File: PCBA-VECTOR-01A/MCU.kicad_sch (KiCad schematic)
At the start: 24 parts, among them J12 Conn_02x03_Odd_Even, U11 STM32G473RCTx, Y1 25MHz, Y2 32.768kHz

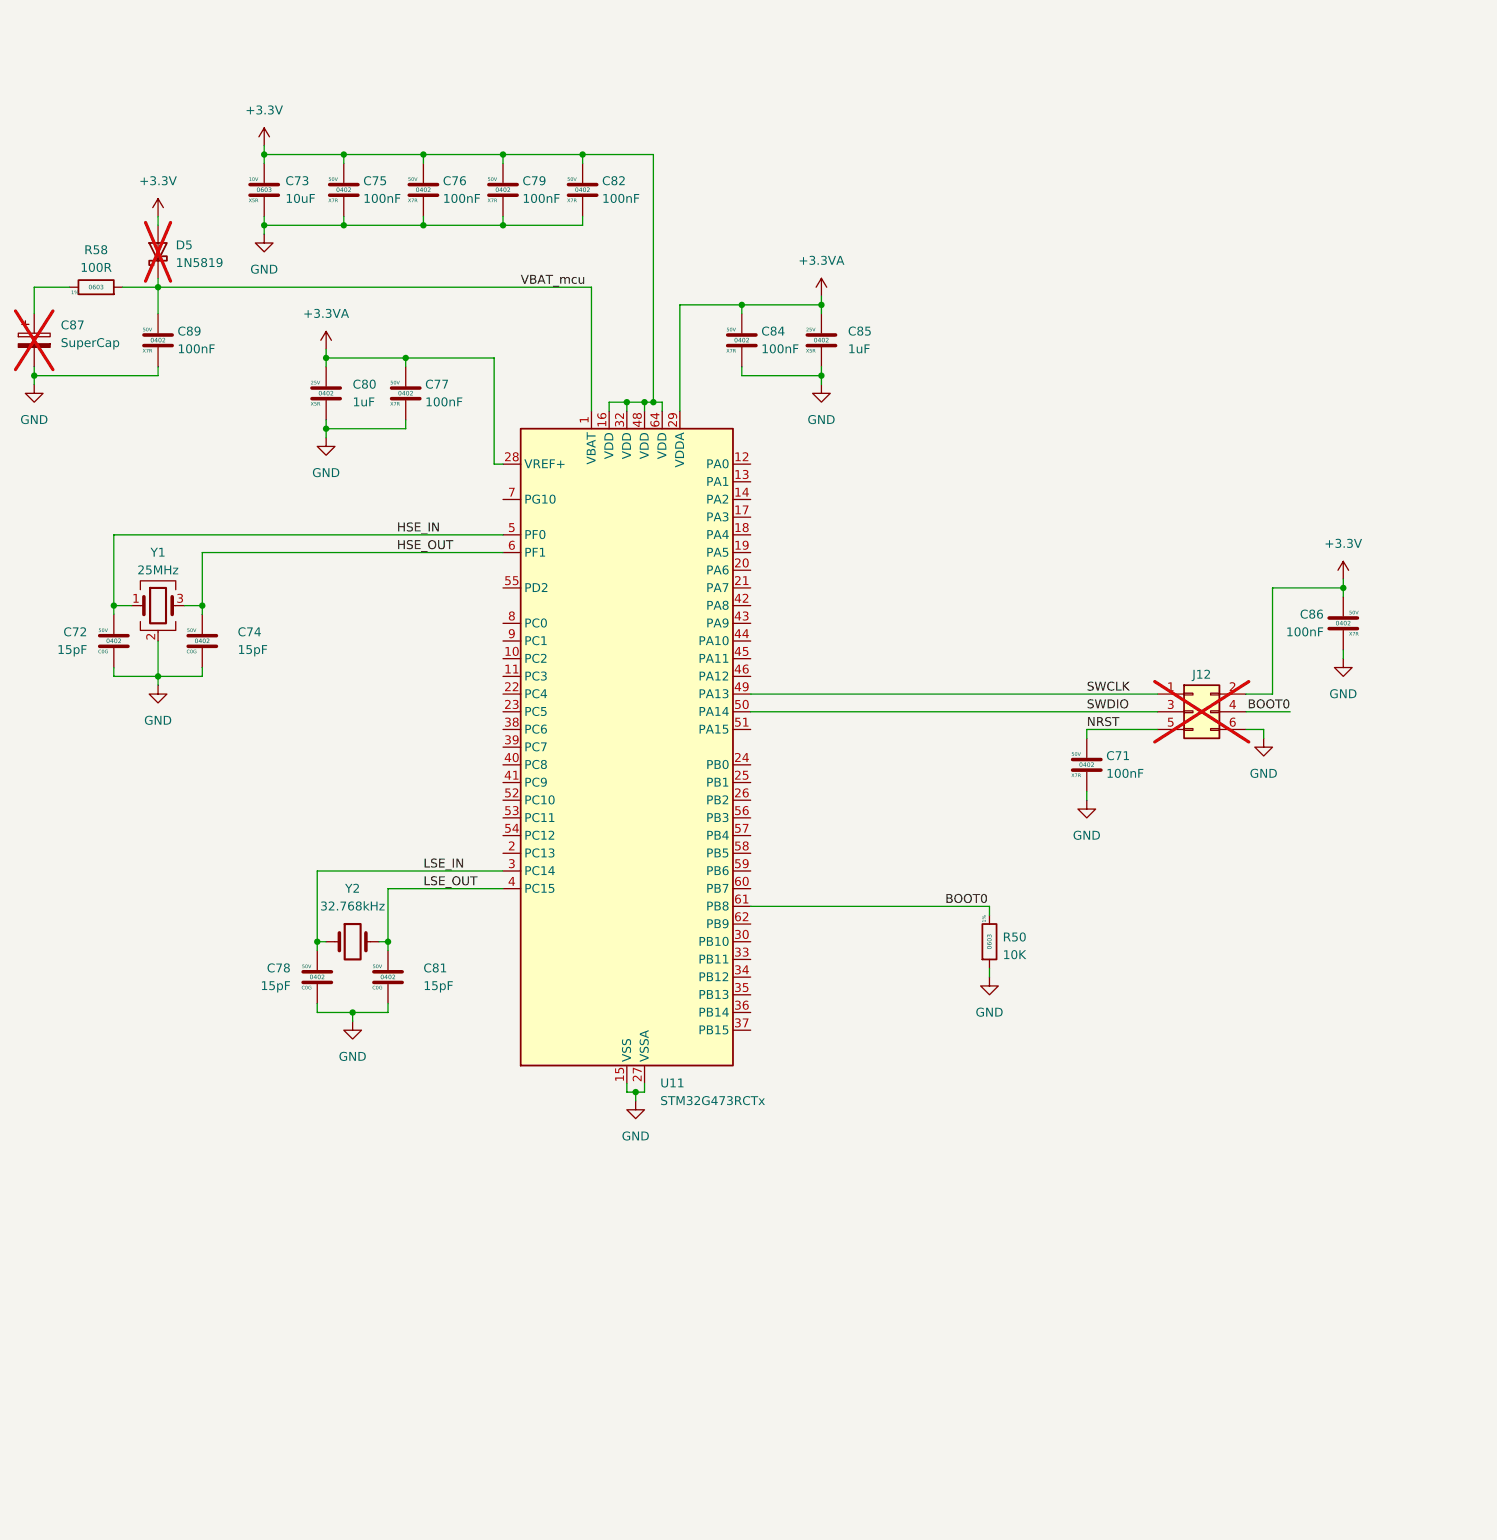
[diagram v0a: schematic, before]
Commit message: Changes were made
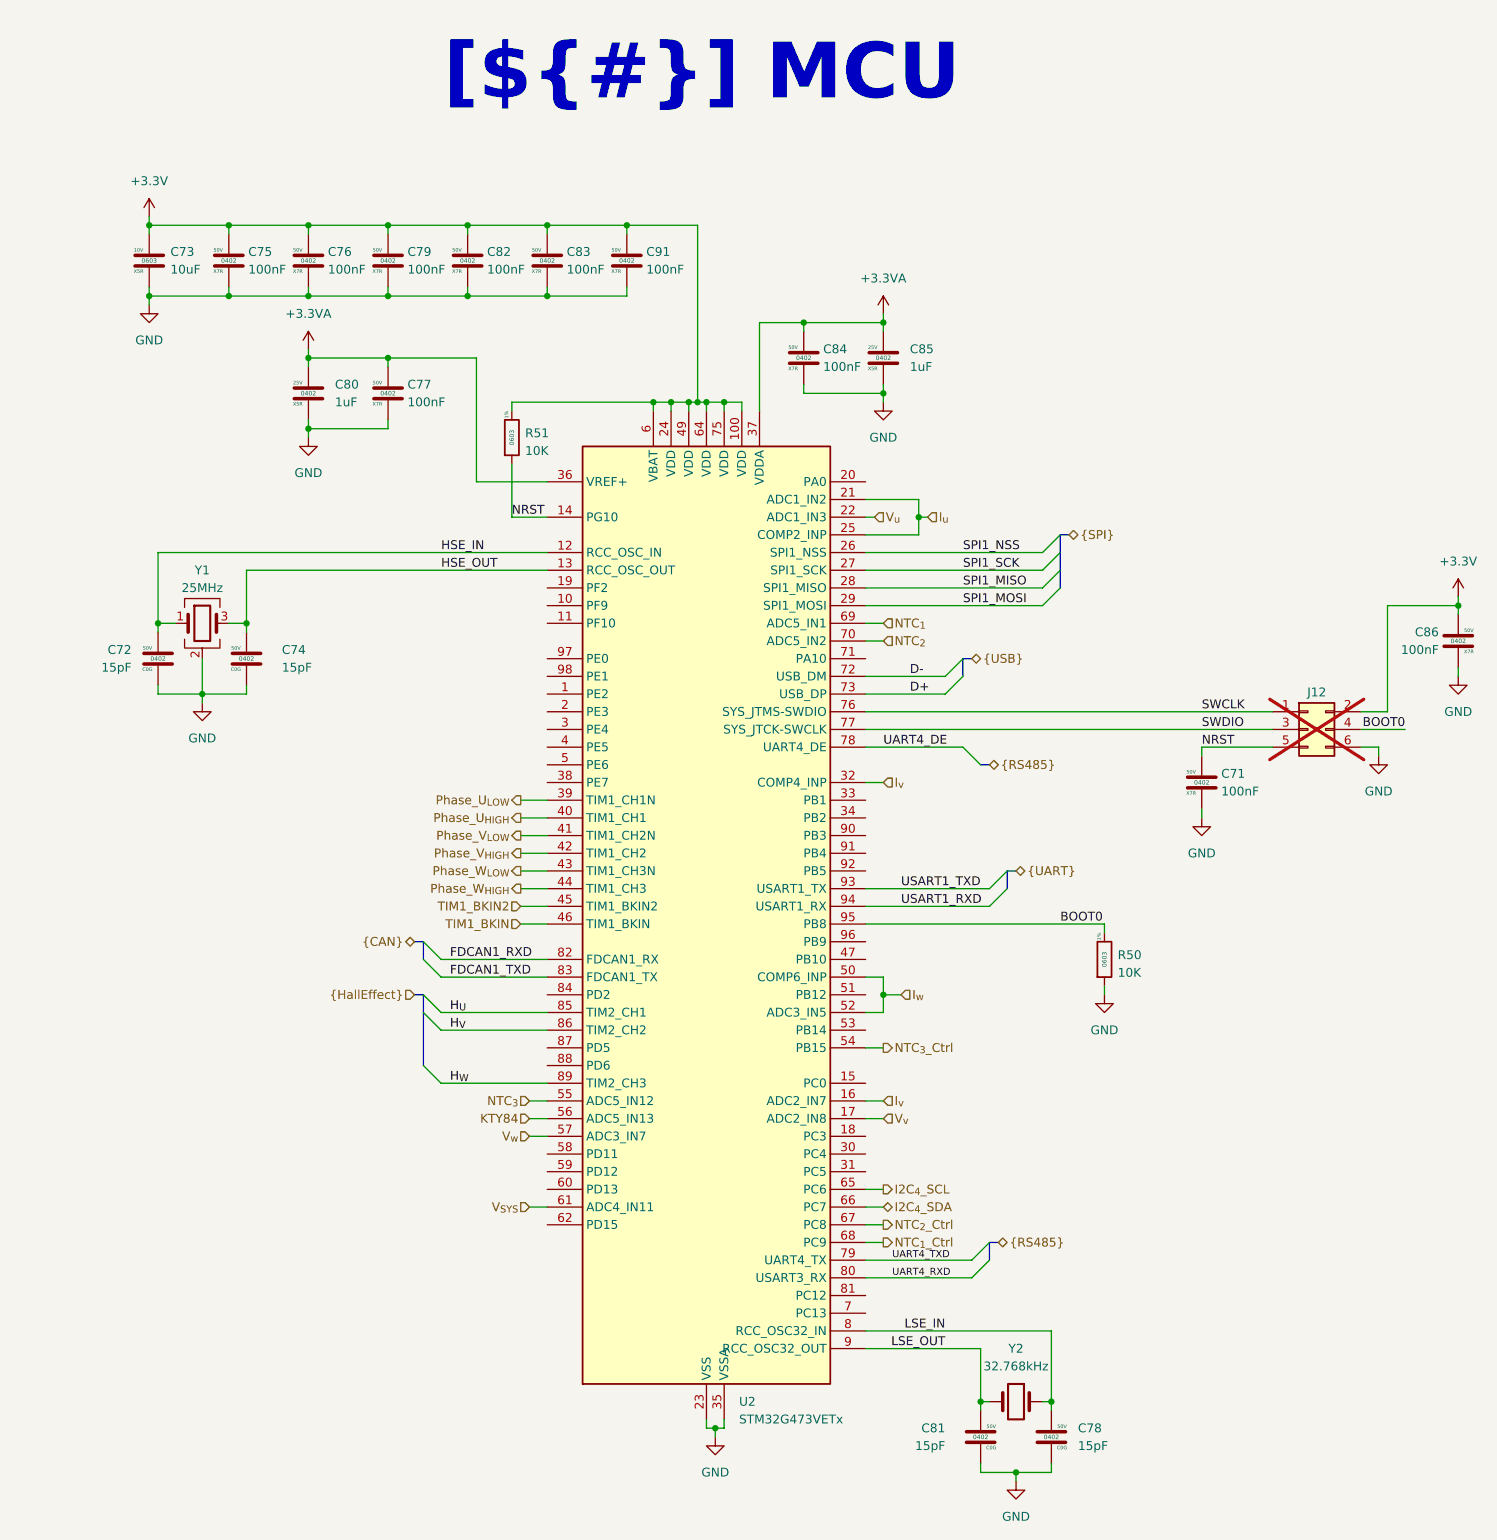
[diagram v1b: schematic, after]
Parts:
- removed C87: SuperCap, Capacitor_THT:C_Rect_L7.2mm_W11.0mm_P5.00mm_FKS2_FKP2_MKS2_MKP2, symbol Device:C_Polarized
- removed C89: 100nF, Capacitor_SMD:C_0402_1005Metric, symbol Device:C
- removed D5: 1N5819, Diode_THT:D_DO-41_SOD81_P10.16mm_Horizontal, symbol Diode:1N5819
- removed R58: 100R, Resistor_SMD:R_0603_1608Metric, symbol Device:R
- removed U11: STM32G473RCTx, Package_QFP:LQFP-64_10x10mm_P0.5mm, symbol MCU_ST_STM32G4:STM32G473RCTx
- added C83, C91: 100nF, Capacitor_SMD:C_0402_1005Metric, symbol Device:C
- added R51: 10K, Resistor_SMD:R_0603_1608Metric, symbol Device:R
- added U2: STM32G473VETx, Package_QFP:LQFP-100_14x14mm_P0.5mm, symbol MCU_ST_STM32G4:STM32G473VETx
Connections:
- net +3.3V: now also C83.1, C91.1, R51.1, U2.100 (VDD), U2.24 (VDD), U2.49 (VDD), U2.6 (VBAT), U2.64 (VDD), U2.75 (VDD)
- net +3.3VA: now also U2.36 (VREF+), U2.37 (VDDA)
- net BOOT0: now also U2.95 (PB8)
- net GND: now also C83.2, C91.2, U2.23 (VSS), U2.35 (VSSA), U2.48 (VSS), U2.63 (VSS), U2.74 (VSS), U2.99 (VSS)
- net HSE_IN: now also U2.12 (PF0)
- net HSE_OUT: now also U2.13 (PF1)
- net LSE_IN: now also U2.8 (PC14)
- net LSE_OUT: now also U2.9 (PC15)
- net NRST: now also R51.2, U2.14 (PG10)
- net SWCLK: now also U2.76 (PA13)
- net SWDIO: now also U2.77 (PA14)
- new net D+: U2.73 (PA12)
- new net D-: U2.72 (PA11)
- new net FDCAN1_RXD: U2.82 (PD0)
- new net FDCAN1_TXD: U2.83 (PD1)
- new net H_{U}: U2.85 (PD3)
- new net H_{V}: U2.86 (PD4)
- new net H_{W}: U2.89 (PD7)
- new net I2C_{4}_SCL: U2.65 (PC6)
- new net I2C_{4}_SDA: U2.66 (PC7)
- new net I_{u}: U2.21 (PA1), U2.25 (PA3)
- new net I_{v}: U2.16 (PC1), U2.32 (PB0)
- new net I_{w}: U2.50 (PB11), U2.52 (PB13)
- new net KTY84: U2.56 (PD9)
- new net NTC_{1}: U2.69 (PA8)
- new net NTC_{1}_Ctrl: U2.68 (PC9)
- new net NTC_{2}: U2.70 (PA9)
- new net NTC_{2}_Ctrl: U2.67 (PC8)
- new net NTC_{3}: U2.55 (PD8)
- new net NTC_{3}_Ctrl: U2.54 (PB15)
- new net Phase_U_{HIGH}: U2.40 (PE9)
- new net Phase_U_{LOW}: U2.39 (PE8)
- new net Phase_V_{HIGH}: U2.42 (PE11)
- new net Phase_V_{LOW}: U2.41 (PE10)
- new net Phase_W_{HIGH}: U2.44 (PE13)
- new net Phase_W_{LOW}: U2.43 (PE12)
- new net SPI1_MISO: U2.28 (PA6)
- new net SPI1_MOSI: U2.29 (PA7)
- new net SPI1_NSS: U2.26 (PA4)
- new net SPI1_SCK: U2.27 (PA5)
- new net TIM1_BKIN: U2.46 (PE15)
- new net TIM1_BKIN2: U2.45 (PE14)
- new net UART4_DE: U2.78 (PA15)
- new net UART4_RXD: U2.80 (PC11)
- new net UART4_TXD: U2.79 (PC10)
- new net USART1_RXD: U2.94 (PB7)
- new net USART1_TXD: U2.93 (PB6)
- new net V_{SYS}: U2.61 (PD14)
- new net V_{u}: U2.22 (PA2)
- new net V_{v}: U2.17 (PC2)
- new net V_{w}: U2.57 (PD10)
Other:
- company: (none) -> Jovanovski Laboratory - JLab
- moved on the sheet: C71, C72, C73, C74, C75, C76, C77, C78, C79, C80, C81, C82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
